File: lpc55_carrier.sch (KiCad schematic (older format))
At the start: 49 parts, among them J101 Conn_2Rows-51Pins, U101 LPC55S28JBD64, Y101 16MHz, Y102 32.768kHz

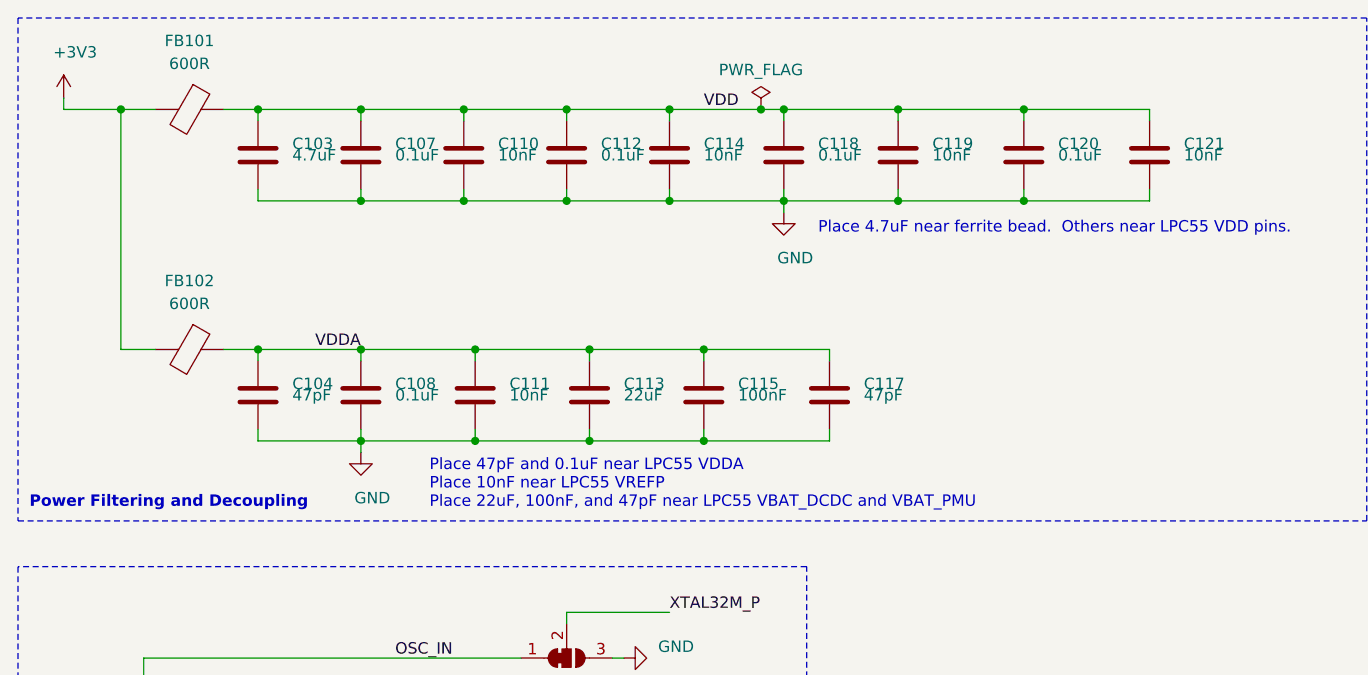
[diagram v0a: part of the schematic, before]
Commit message: lpc55_carrier: add 4.7uF bulk cap to VDDA
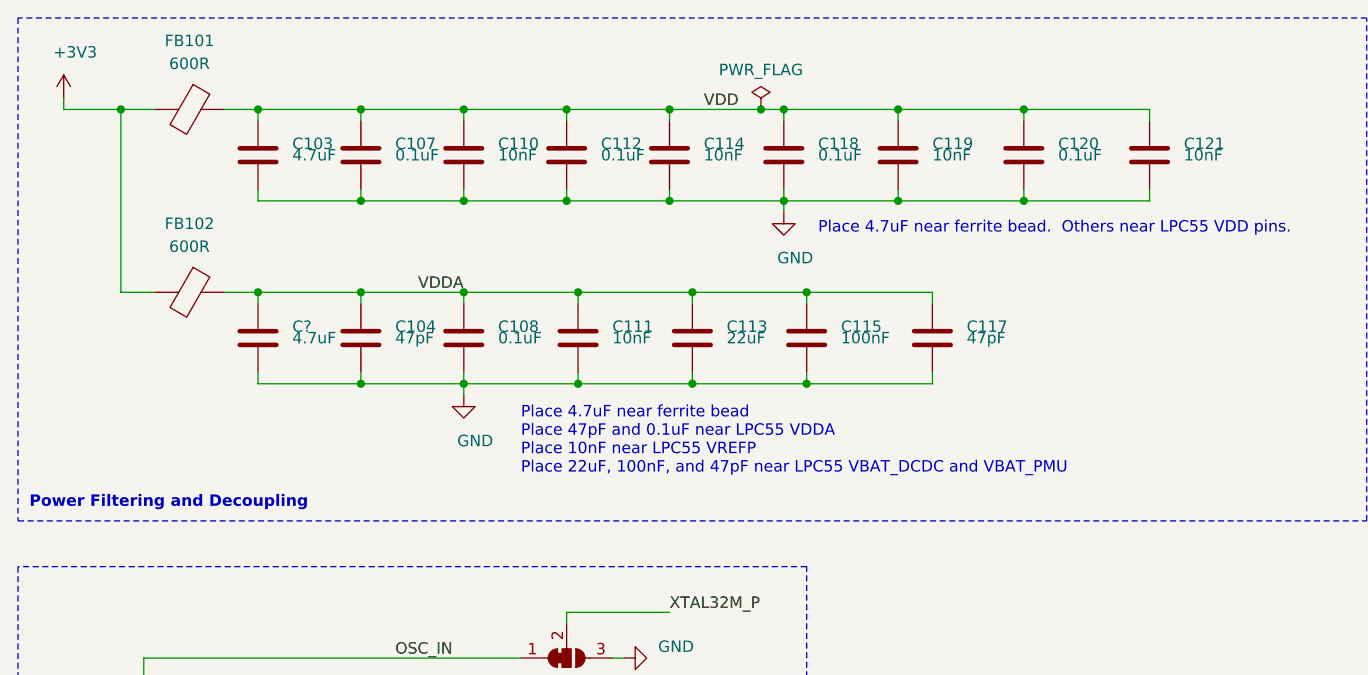
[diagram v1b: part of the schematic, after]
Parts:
- added C?: 4.7uF, Capacitor_SMD:C_0603_1608Metric, symbol Device:C
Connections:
- net GND: now also C?.2
- net VDDA: now also C?.1
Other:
- note added: "Place 4.7uF near ferrite bead\nPlace 47pF and 0.1uF near LPC55 VDDA\nPlace 10nF near LPC55 VREFP\nPlace 22uF, 100nF, and 47pF near LPC55 VBAT_DCDC and VBAT_PMU"
- note removed: "Place 47pF and 0.1uF near LPC55 VDDA\nPlace 10nF near LPC55 VREFP\nPlace 22uF, 100nF, and 47pF near LPC55 VBAT_DCDC and VBAT_PMU"
- moved on the sheet: C104, C108, C111, C113, C115, C117, FB102
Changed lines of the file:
@@
 L Device:Ferrite_Bead FB102
 U 1 1 5F378364
-P 1950 2800
-F 0 "FB102" V 1650 2800 50  0000 C CNN
-F 1 "600R" V 1750 2800 50  0000 C CNN
-F 2 "Inductor_SMD:L_0603_1608Metric" V 1880 2800 50  0001 C CNN
-F 3 "~" H 1950 2800 50  0001 C CNN
-	1    1950 2800
+P 1950 2550
+F 0 "FB102" V 1650 2550 50  0000 C CNN
+F 1 "600R" V 1750 2550 50  0000 C CNN
+F 2 "Inductor_SMD:L_0603_1608Metric" V 1880 2550 50  0001 C CNN
+F 3 "~" H 1950 2550 50  0001 C CNN
+	1    1950 2550
 	0    1    1    0
 $EndComp
 Wire Wire Line
-	1800 2800 1650 2800
-Wire Wire Line
-	1650 2800 1650 1750
+	1800 2550 1650 2550
+Wire Wire Line
+	1650 2550 1650 1750
 Connection ~ 1650 1750
 Wire Wire Line
@@
 L Device:C C104
 U 1 1 5F37DDF6
-P 2250 3000
-F 0 "C104" H 2400 3050 50  0000 L CNN
-F 1 "47pF" H 2400 3000 50  0000 L CNN
-F 2 "Capacitor_SMD:C_0603_1608Metric" H 2288 2850 50  0001 C CNN
-F 3 "~" H 2250 3000 50  0001 C CNN
-	1    2250 3000
+P 2700 2750
+F 0 "C104" H 2850 2800 50  0000 L CNN
+F 1 "47pF" H 2850 2750 50  0000 L CNN
+F 2 "Capacitor_SMD:C_0603_1608Metric" H 2738 2600 50  0001 C CNN
+F 3 "~" H 2700 2750 50  0001 C CNN
+	1    2700 2750
 	1    0    0    -1
 $EndComp
@@
 L Device:C C108
 U 1 1 5F37E1AF
-P 2700 3000
-F 0 "C108" H 2850 3050 50  0000 L CNN
-F 1 "0.1uF" H 2850 3000 50  0000 L CNN
-F 2 "Capacitor_SMD:C_0603_1608Metric" H 2738 2850 50  0001 C CNN
-F 3 "~" H 2700 3000 50  0001 C CNN
-	1    2700 3000
+P 3150 2750
+F 0 "C108" H 3300 2800 50  0000 L CNN
+F 1 "0.1uF" H 3300 2750 50  0000 L CNN
+F 2 "Capacitor_SMD:C_0603_1608Metric" H 3188 2600 50  0001 C CNN
+F 3 "~" H 3150 2750 50  0001 C CNN
+	1    3150 2750
 	1    0    0    -1
 $EndComp
@@
 L Device:C C111
 U 1 1 5F37E466
-P 3200 3000
-F 0 "C111" H 3350 3050 50  0000 L CNN
-F 1 "10nF" H 3350 3000 50  0000 L CNN
-F 2 "Capacitor_SMD:C_0603_1608Metric" H 3238 2850 50  0001 C CNN
-F 3 "~" H 3200 3000 50  0001 C CNN
-	1    3200 3000
+P 3650 2750
+F 0 "C111" H 3800 2800 50  0000 L CNN
+F 1 "10nF" H 3800 2750 50  0000 L CNN
+F 2 "Capacitor_SMD:C_0603_1608Metric" H 3688 2600 50  0001 C CNN
+F 3 "~" H 3650 2750 50  0001 C CNN
+	1    3650 2750
 	1    0    0    -1
 $EndComp
@@
 L power:GND #PWR0106
 U 1 1 5F37E83A
-P 2700 3250
-F 0 "#PWR0106" H 2700 3000 50  0001 C CNN
-F 1 "GND" H 2750 3050 50  0000 C CNN
-F 2 "" H 2700 3250 50  0001 C CNN
-F 3 "" H 2700 3250 50  0001 C CNN
-	1    2700 3250
-	1    0    0    -1
-$EndComp
-Wire Wire Line
-	2100 2800 2250 2800
-Wire Wire Line
-	3200 2800 3200 2850
-Wire Wire Line
-	3200 3150 3200 3200
-Wire Wire Line
-	3200 3200 2700 3200
-Wire Wire Line
-	2250 3200 2250 3150
-Wire Wire Line
-	2700 3250 2700 3200
-Connection ~ 2700 3200
-Wire Wire Line
-	2700 3200 2250 3200
-Wire Wire Line
-	2700 3200 2700 3150
-Wire Wire Line
-	2700 2850 2700 2800
-Connection ~ 2700 2800
-Wire Wire Line
-	2700 2800 3200 2800
-Wire Wire Line
-	2250 2850 2250 2800
-Connection ~ 2250 2800
-Wire Wire Line
-	2250 2800 2700 2800
-Text Label 2500 2800 0    50   ~ 0
+P 3150 3000
+F 0 "#PWR0106" H 3150 2750 50  0001 C CNN
+F 1 "GND" H 3200 2800 50  0000 C CNN
+F 2 "" H 3150 3000 50  0001 C CNN
+F 3 "" H 3150 3000 50  0001 C CNN
+	1    3150 3000
+	1    0    0    -1
+$EndComp
+Wire Wire Line
+	2100 2550 2250 2550
+Wire Wire Line
+	3650 2550 3650 2600
+Wire Wire Line
+	3650 2900 3650 2950
+Wire Wire Line
+	3650 2950 3150 2950
+Wire Wire Line
+	2700 2950 2700 2900
+Wire Wire Line
+	3150 3000 3150 2950
+Connection ~ 3150 2950
+Wire Wire Line
+	3150 2950 2700 2950
+Wire Wire Line
+	3150 2950 3150 2900
+Wire Wire Line
+	3150 2600 3150 2550
+Connection ~ 3150 2550
+Wire Wire Line
+	3150 2550 3650 2550
+Wire Wire Line
+	2700 2600 2700 2550
+Connection ~ 2700 2550
+Wire Wire Line
+	2700 2550 3150 2550
+Text Label 2950 2550 0    50   ~ 0
 VDDA
 Text Notes 4700 2300 0    50   ~ 0
 Place 4.7uF near ferrite bead.  Others near LPC55 VDD pins.
-Text Notes 3000 3500 0    50   ~ 0
-Place 47pF and 0.1uF near LPC55 VDDA\nPlace 10nF near LPC55 VREFP\nPlace 22uF, 100nF, and 47pF near LPC55 VBAT_DCDC and VBAT_PMU
+Text Notes 3400 3350 0    50   ~ 0
+Place 4.7uF near ferrite bead\nPlace 47pF and 0.1uF near LPC55 VDDA\nPlace 10nF near LPC55 VREFP\nPlace 22uF, 100nF, and 47pF near LPC55 VBAT_DCDC and VBAT_PMU
 Wire Notes Line
 	1200 1350 1200 3550
@@
 L Device:C C113
 U 1 1 5F382DA2
-P 3700 3000
-F 0 "C113" H 3850 3050 50  0000 L CNN
-F 1 "22uF" H 3850 3000 50  0000 L CNN
-F 2 "Capacitor_SMD:C_0805_2012Metric" H 3738 2850 50  0001 C CNN
-F 3 "~" H 3700 3000 50  0001 C CNN
-	1    3700 3000
+P 4150 2750
+F 0 "C113" H 4300 2800 50  0000 L CNN
+F 1 "22uF" H 4300 2750 50  0000 L CNN
+F 2 "Capacitor_SMD:C_0805_2012Metric" H 4188 2600 50  0001 C CNN
+F 3 "~" H 4150 2750 50  0001 C CNN
+	1    4150 2750
 	1    0    0    -1
 $EndComp
@@
 L Device:C C115
 U 1 1 5F3830C2
-P 4200 3000
-F 0 "C115" H 4350 3050 50  0000 L CNN
-F 1 "100nF" H 4350 3000 50  0000 L CNN
-F 2 "Capacitor_SMD:C_0603_1608Metric" H 4238 2850 50  0001 C CNN
-F 3 "~" H 4200 3000 50  0001 C CNN
-	1    4200 3000
+P 4650 2750
+F 0 "C115" H 4800 2800 50  0000 L CNN
+F 1 "100nF" H 4800 2750 50  0000 L CNN
+F 2 "Capacitor_SMD:C_0603_1608Metric" H 4688 2600 50  0001 C CNN
+F 3 "~" H 4650 2750 50  0001 C CNN
+	1    4650 2750
 	1    0    0    -1
 $EndComp
@@
 L Device:C C117
 U 1 1 5F3834EB
-P 4750 3000
-F 0 "C117" H 4900 3050 50  0000 L CNN
-F 1 "47pF" H 4900 3000 50  0000 L CNN
-F 2 "Capacitor_SMD:C_0603_1608Metric" H 4788 2850 50  0001 C CNN
-F 3 "~" H 4750 3000 50  0001 C CNN
-	1    4750 3000
-	1    0    0    -1
-$EndComp
-Wire Wire Line
-	3200 3200 3700 3200
-Wire Wire Line
-	4750 3200 4750 3150
-Connection ~ 3200 3200
-Wire Wire Line
-	4200 3200 4200 3150
-Connection ~ 4200 3200
-Wire Wire Line
-	4200 3200 4750 3200
-Wire Wire Line
-	3700 3150 3700 3200
-Connection ~ 3700 3200
-Wire Wire Line
-	3700 3200 4200 3200
-Wire Wire Line
-	3200 2800 3700 2800
-Wire Wire Line
-	4750 2800 4750 2850
-Connection ~ 3200 2800
-Wire Wire Line
-	4200 2800 4200 2850
-Connection ~ 4200 2800
-Wire Wire Line
-	4200 2800 4750 2800
-Wire Wire Line
-	3700 2800 3700 2850
-Connection ~ 3700 2800
-Wire Wire Line
-	3700 2800 4200 2800
+P 5200 2750
+F 0 "C117" H 5350 2800 50  0000 L CNN
+F 1 "47pF" H 5350 2750 50  0000 L CNN
+F 2 "Capacitor_SMD:C_0603_1608Metric" H 5238 2600 50  0001 C CNN
+F 3 "~" H 5200 2750 50  0001 C CNN
+	1    5200 2750
+	1    0    0    -1
+$EndComp
+Wire Wire Line
+	3650 2950 4150 2950
+Wire Wire Line
+	5200 2950 5200 2900
+Connection ~ 3650 2950
+Wire Wire Line
+	4650 2950 4650 2900
+Connection ~ 4650 2950
+Wire Wire Line
+	4650 2950 5200 2950
+Wire Wire Line
+	4150 2900 4150 2950
+Connection ~ 4150 2950
+Wire Wire Line
+	4150 2950 4650 2950
+Wire Wire Line
+	3650 2550 4150 2550
+Wire Wire Line
+	5200 2550 5200 2600
+Connection ~ 3650 2550
+Wire Wire Line
+	4650 2550 4650 2600
+Connection ~ 4650 2550
+Wire Wire Line
+	4650 2550 5200 2550
+Wire Wire Line
+	4150 2550 4150 2600
+Connection ~ 4150 2550
+Wire Wire Line
+	4150 2550 4650 2550
 Wire Wire Line
 	12000 2500 12200 2500
@@
 Wire Wire Line
 	4450 1750 4550 1750
+$Comp
+L Device:C C?
+U 1 1 5F7DE78D
+P 2250 2750
+F 0 "C?" H 2400 2800 50  0000 L CNN
+F 1 "4.7uF" H 2400 2750 50  0000 L CNN
+F 2 "Capacitor_SMD:C_0603_1608Metric" H 2288 2600 50  0001 C CNN
+F 3 "~" H 2250 2750 50  0001 C CNN
+	1    2250 2750
+	1    0    0    -1
+$EndComp
+Wire Wire Line
+	2250 2600 2250 2550
+Connection ~ 2250 2550
+Wire Wire Line
+	2250 2550 2700 2550
+Wire Wire Line
+	2250 2900 2250 2950
+Wire Wire Line
+	2250 2950 2700 2950
+Connection ~ 2700 2950
 $EndSCHEMATC
